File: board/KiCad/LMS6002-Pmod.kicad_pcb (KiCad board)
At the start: 2 copper layers, 30.5 x 29.2 mm, 3 parts, among them P1 PMOD_2x6, P2 PMOD_2x6, U1 iCE40_1K4K_TQ144

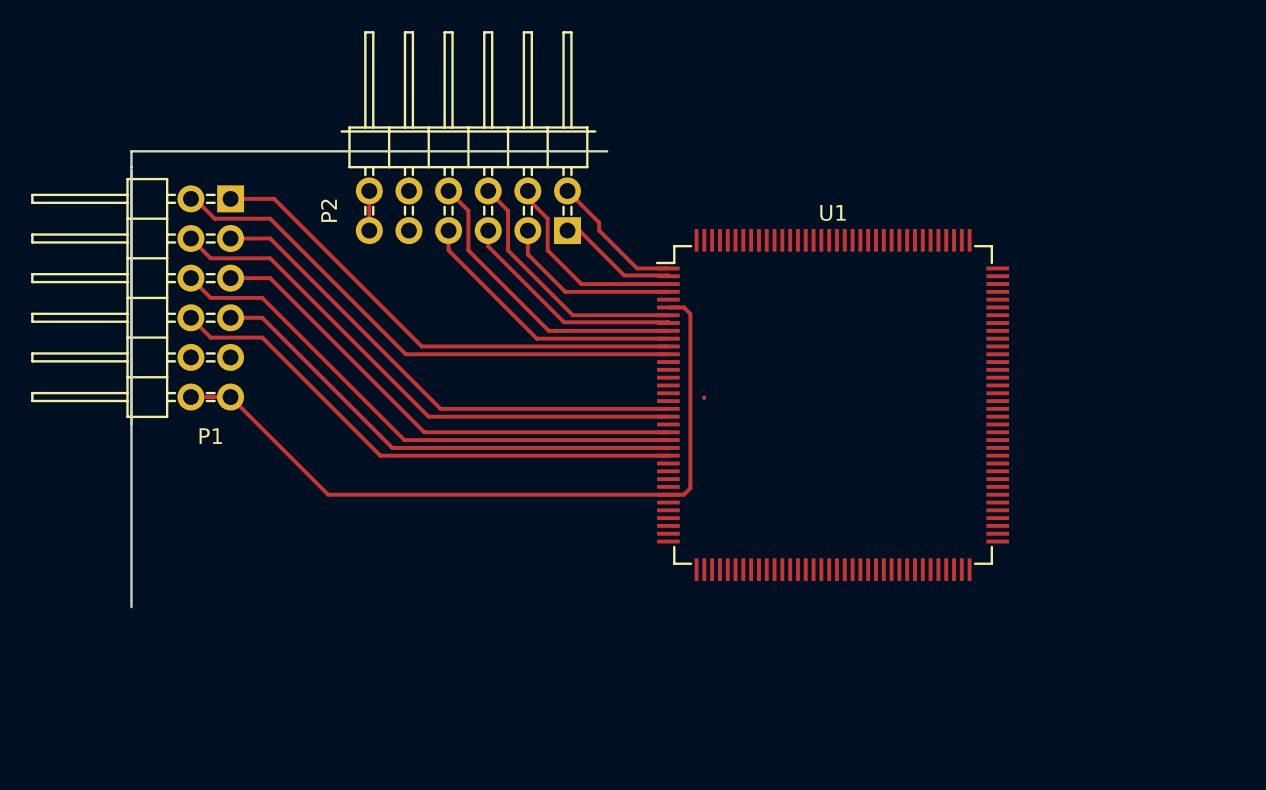
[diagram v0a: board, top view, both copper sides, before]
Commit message: Finalize first draft
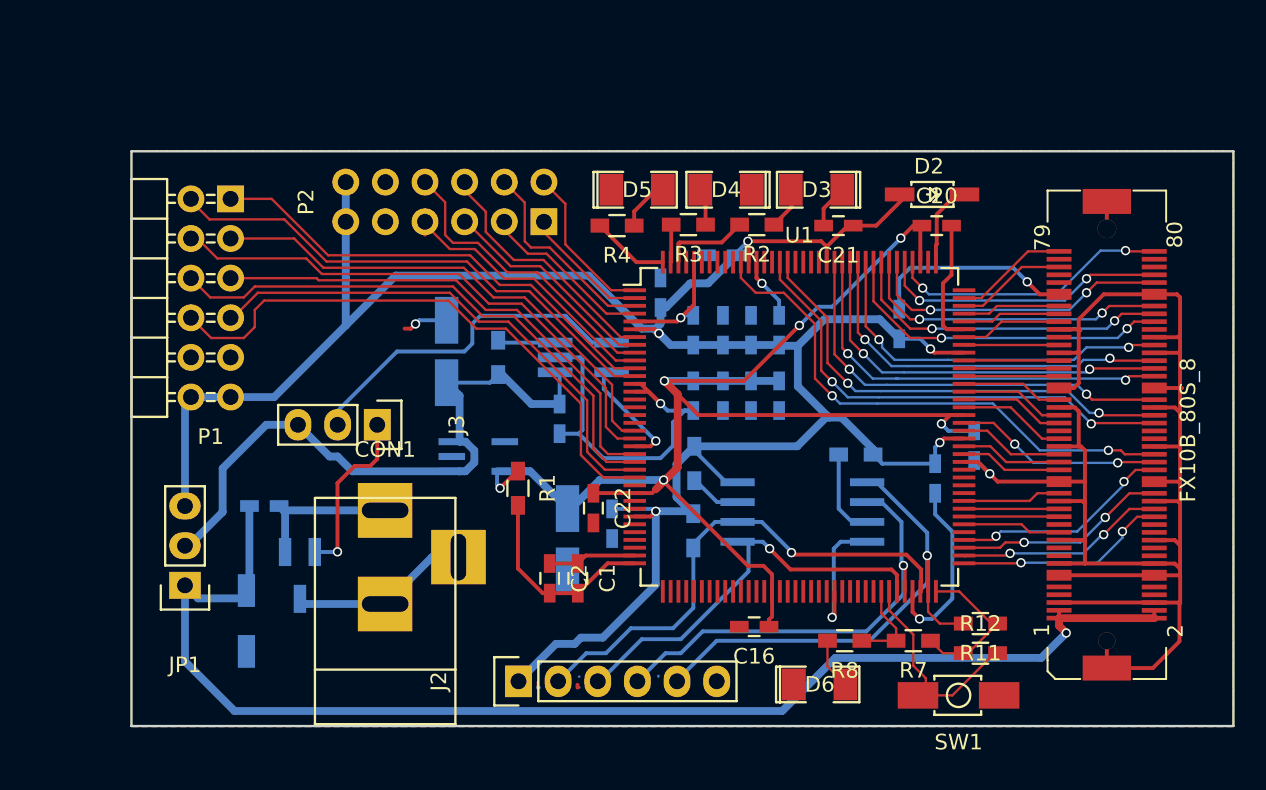
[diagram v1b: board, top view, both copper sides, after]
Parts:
- added C1: 10µF, Capacitors_SMD:C_0603_HandSoldering, F.Cu at (117.5, 112.2)
- added C10: 10µF, Capacitors_SMD:C_0603_HandSoldering, B.Cu at (126.8, 96.3)
- added C11: 1µF, Capacitors_SMD:C_0603_HandSoldering, B.Cu at (128.6, 96.3)
- added C12: 0.1µF, Capacitors_SMD:C_0603_HandSoldering, B.Cu at (130.4, 96.3)
- added C13: 0.01µF, Capacitors_SMD:C_0603_HandSoldering, B.Cu at (124.9, 96.3)
- added C14: 100n, Capacitors_SMD:C_0603_HandSoldering, B.Cu at (140.4, 105.8)
- added C15: 100n, Capacitors_SMD:C_0603_HandSoldering, B.Cu at (122.8, 93.9)
- added C16: 100n, Capacitors_SMD:C_0603_HandSoldering, F.Cu at (128.8, 115.3)
- added C17: 100n, Capacitors_SMD:C_0603_HandSoldering, B.Cu at (119.7, 108.7)
- added C18: 100n, Capacitors_SMD:C_0603_HandSoldering, B.Cu at (142.9, 103.7)
- added C19: 100n, Capacitors_SMD:C_0603_HandSoldering, B.Cu at (138.1, 95.9)
- added C2: 0.1µF, Capacitors_SMD:C_0603_HandSoldering, F.Cu at (115.7, 112.2)
- added C20: 100n, Capacitors_SMD:C_0603_HandSoldering, F.Cu at (140.5, 89.6)
- added C21: 100n, Capacitors_SMD:C_0603_HandSoldering, F.Cu at (134.2, 89.6)
- added C22: 100n, Capacitors_SMD:C_0603_HandSoldering, F.Cu at (118.5, 107.7)
- added C23: 100n, Capacitors_SMD:C_0603_HandSoldering, B.Cu at (126.7, 91.5)
- added C3: 1µF, Capacitors_Tantalum_SMD:TantalC_SizeA_EIA-3216_HandSoldering, B.Cu at (109.1, 97.7)
- added C4: 1µF, Capacitors_Tantalum_SMD:TantalC_SizeA_EIA-3216_HandSoldering, B.Cu at (116.8, 109.7)
- added C5: 0.1µ, Capacitors_SMD:C_0603_HandSoldering, B.Cu at (116.3, 102.0)
- added C6: 10µF, Capacitors_SMD:C_0603_HandSoldering, B.Cu at (126.8, 100.5)
- added C7: 1µF, Capacitors_SMD:C_0603_HandSoldering, B.Cu at (128.6, 100.5)
- added C8: 0.1µF, Capacitors_SMD:C_0603_HandSoldering, B.Cu at (124.9, 100.5)
- added C9: 0.01µF, Capacitors_SMD:C_0603_HandSoldering, B.Cu at (130.4, 100.5)
- added CON1: BARREL_JACK, Connect:BARREL_JACK, F.Cu at (105.2, 114.0)
- added D1: 5V-SOD-123F, pmod:SOD-123F_Handsoldering, B.Cu at (96.3, 114.9)
- added D2: Schottky 0520, pmod:SOD-123_Handsoldering, F.Cu at (140.2, 87.6)
- added D3: LED, SMD_Packages:SMD-1206_Pol, F.Cu at (132.8, 87.3)
- added D4: LED, SMD_Packages:SMD-1206_Pol, F.Cu at (127.0, 87.3)
- added D5: LED, SMD_Packages:SMD-1206_Pol, F.Cu at (121.3, 87.3)
- added D6: LED, SMD_Packages:SMD-1206_Pol, F.Cu at (133.0, 119.0)
- added F1: 2A-0603, Capacitors_SMD:C_0603_HandSoldering, B.Cu at (97.4, 107.6)
- added J1: FX10B_80S_8, pmod:FX10B_80S_8, F.Cu at (151.4, 103.0)
- added J2: Pinheader_1x6_TH, Pin_Headers:Pin_Header_Straight_1x06, F.Cu at (113.7, 118.8)
- added J3: SELECT_DIV, Pin_Headers:Pin_Header_Straight_1x03, F.Cu at (104.6, 102.4)
- added JP1: LDO_1V2_IN_SEL, Pin_Headers:Pin_Header_Straight_1x03, F.Cu at (92.3, 112.6)
- added Q1: IRLML6344bpf, TO_SOT_Packages_SMD:SOT-23_Handsoldering, B.Cu at (99.7, 112.0)
- added R1: 100, Resistors_SMD:R_0603_HandSoldering, F.Cu at (113.7, 106.4)
- added R10: 10k, Resistors_SMD:R_0603_HandSoldering, B.Cu at (135.3, 104.3)
- added R11: 10k, Resistors_SMD:R_0603_HandSoldering, F.Cu at (143.3, 115.1)
- added R12: 10K, Resistors_SMD:R_0603_HandSoldering, F.Cu at (143.3, 117.0)
- added R2: 10, Resistors_SMD:R_0603_HandSoldering, F.Cu at (129.0, 89.5)
- added R3: 10, Resistors_SMD:R_0603_HandSoldering, F.Cu at (124.6, 89.5)
- added R4: 10, Resistors_SMD:R_0603_HandSoldering, F.Cu at (120.0, 89.6)
- added R5: R, Resistors_SMD:R_0603_HandSoldering, B.Cu at (112.4, 98.0)
- added R6: 10k, Resistors_SMD:R_0603_HandSoldering, B.Cu at (124.9, 109.2)
- added R7: 10K, Resistors_SMD:R_0603_HandSoldering, F.Cu at (139.0, 116.2)
- added R8: 10, Resistors_SMD:R_0603_HandSoldering, F.Cu at (134.6, 116.2)
- added R9: 10k, Resistors_SMD:R_0603_HandSoldering, B.Cu at (125.0, 104.8)
- added SW1: ICE_RESET, pmod:B3U-1000P_Handsoldering, F.Cu at (141.9, 119.7)
- added U2: LD6815, pmod:SOT-753_(TSOP-5)_Handsoldering, B.Cu at (111.1, 104.4)
- added U3: LTC1799, pmod:TSOT-23_Handsoldering, B.Cu at (117.9, 98.0)
- added U4: N25Q, pmod:SOP2-8_Handsoldering, B.Cu at (131.9, 108.0)
- moved U1 2.57 mm to (131.7, 102.5)
- moved P2 1.61 mm to (116.6, 83.0)
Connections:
- P1 pad 12: +3V3 -> 3V3_PMOD
- P1 pad 6: +3V3 -> 3V3_PMOD
- P2 pad 12: +3V3 -> 3V3_PMOD
- P2 pad 6: +3V3 -> 3V3_PMOD
- U1 pad 100: Net-(U1-Pad100) -> 3V3_PMOD
- U1 pad 101: Net-(U1-Pad101) -> FCLK2
- U1 pad 102: Net-(U1-Pad102) -> RFDIO_GPIO0
- U1 pad 103: Net-(U1-Pad103) -> GND
- U1 pad 104: Net-(U1-Pad104) -> RFDIO_GPIO1
- U1 pad 105: Net-(U1-Pad105) -> RFDIO_GPIO2
- U1 pad 106: Net-(U1-Pad106) -> RFDIO_REF_CLK_IN
- U1 pad 107: Net-(U1-Pad107) -> TXEN
- U1 pad 108: Net-(U1-Pad108) -> (no net)
- U1 pad 110: Net-(U1-Pad110) -> (no net)
- U1 pad 111: Net-(U1-Pad111) -> 1V2_LDO
- U1 pad 112: Net-(U1-Pad112) -> RXEN
- U1 pad 113: Net-(U1-Pad113) -> RFDIO_SPI_EN
- U1 pad 114: Net-(U1-Pad114) -> RFDIO_SPI_CLK
- U1 pad 115: Net-(U1-Pad115) -> RFDIO_SPI_MISO
- U1 pad 116: Net-(U1-Pad116) -> RFDIO_SPI_MOSI
- U1 pad 117: Net-(U1-Pad117) -> RFDIO_RESET
- U1 pad 118: Net-(U1-Pad118) -> FCLK1
- U1 pad 119: Net-(U1-Pad119) -> DIQ2_D11
- U1 pad 120: Net-(U1-Pad120) -> DIQ2_D9
- U1 pad 121: Net-(U1-Pad121) -> DIQ2_D7
- U1 pad 122: Net-(U1-Pad122) -> DIQ2_D5
- U1 pad 123: Net-(U1-Pad123) -> 3V3_PMOD
- U1 pad 124: Net-(U1-Pad124) -> (no net)
- U1 pad 125: Net-(U1-Pad125) -> (no net)
- U1 pad 126: Net-(U1-Pad126) -> (no net)
- U1 pad 127: Net-(U1-Pad127) -> (no net)
- U1 pad 128: Net-(U1-Pad128) -> DIQ2_D3
- U1 pad 129: Net-(U1-Pad129) -> DIQ2_D1
- U1 pad 13: Net-(U1-Pad13) -> GND
- U1 pad 130: Net-(U1-Pad130) -> (no net)
- U1 pad 131: Net-(U1-Pad131) -> (no net)
- U1 pad 132: Net-(U1-Pad132) -> GND
- U1 pad 133: Net-(U1-Pad133) -> 3V3_PMOD
- U1 pad 134: Net-(U1-Pad134) -> DIQ1_D11
- U1 pad 135: Net-(U1-Pad135) -> (no net)
- U1 pad 136: Net-(U1-Pad136) -> (no net)
- U1 pad 137: Net-(U1-Pad137) -> (no net)
- U1 pad 138: Net-(U1-Pad138) -> (no net)
- U1 pad 139: Net-(U1-Pad139) -> (no net)
- U1 pad 14: Net-(U1-Pad14) -> GND
- U1 pad 140: Net-(U1-Pad140) -> GND
- U1 pad 141: Net-(U1-Pad141) -> (no net)
- U1 pad 15: Net-(U1-Pad15) -> (no net)
- U1 pad 16: Net-(U1-Pad16) -> (no net)
- U1 pad 17: Net-(U1-Pad17) -> (no net)
- U1 pad 18: Net-(U1-Pad18) -> (no net)
- U1 pad 21: Net-(U1-Pad21) -> ICE_CLK_IN
- U1 pad 26: Net-(U1-Pad26) -> (no net)
- U1 pad 27: Net-(U1-Pad27) -> 1V2_LDO
- U1 pad 28: Net-(U1-Pad28) -> (no net)
- U1 pad 29: Net-(U1-Pad29) -> (no net)
- U1 pad 30: +3V3 -> 3V3_PMOD
- U1 pad 31: Net-(U1-Pad31) -> (no net)
- U1 pad 32: Net-(U1-Pad32) -> (no net)
- U1 pad 33: Net-(U1-Pad33) -> (no net)
- U1 pad 34: Net-(U1-Pad34) -> (no net)
- U1 pad 37: Net-(U1-Pad37) -> (no net)
- U1 pad 38: Net-(U1-Pad38) -> (no net)
- U1 pad 39: Net-(U1-Pad39) -> (no net)
- U1 pad 40: Net-(U1-Pad40) -> (no net)
- U1 pad 41: Net-(U1-Pad41) -> (no net)
- U1 pad 42: Net-(U1-Pad42) -> (no net)
- U1 pad 43: Net-(U1-Pad43) -> (no net)
- U1 pad 44: Net-(U1-Pad44) -> (no net)
- U1 pad 45: Net-(U1-Pad45) -> (no net)
- U1 pad 46: Net-(U1-Pad46) -> (no net)
- U1 pad 47: Net-(U1-Pad47) -> (no net)
- U1 pad 48: Net-(U1-Pad48) -> (no net)
- U1 pad 49: Net-(U1-Pad49) -> (no net)
- U1 pad 5: Net-(U1-Pad5) -> GND
- U1 pad 50: Net-(U1-Pad50) -> (no net)
- U1 pad 51: Net-(U1-Pad51) -> 1V2_LDO
- U1 pad 52: Net-(U1-Pad52) -> (no net)
- U1 pad 53: Net-(U1-Pad53) -> (no net)
- U1 pad 54: Net-(U1-Pad54) -> (no net)
- U1 pad 55: Net-(U1-Pad55) -> (no net)
- U1 pad 56: Net-(U1-Pad56) -> (no net)
- U1 pad 57: Net-(U1-Pad57) -> (no net)
- U1 pad 58: Net-(U1-Pad58) -> (no net)
- U1 pad 59: Net-(U1-Pad59) -> GND
- U1 pad 6: +3V3 -> 3V3_PMOD
- U1 pad 60: Net-(U1-Pad60) -> (no net)
- U1 pad 61: Net-(U1-Pad61) -> (no net)
- U1 pad 62: Net-(U1-Pad62) -> (no net)
- U1 pad 63: Net-(U1-Pad63) -> (no net)
- U1 pad 64: Net-(U1-Pad64) -> (no net)
- U1 pad 65: Net-(U1-Pad65) -> ICE_CDONE
- U1 pad 66: Net-(U1-Pad66) -> ICE_CRESET_B
- U1 pad 67: Net-(U1-Pad67) -> EXT_SPI_MOSI
- U1 pad 68: Net-(U1-Pad68) -> EXT_SPI_MISO
- U1 pad 69: Net-(U1-Pad69) -> GND
- U1 pad 70: Net-(U1-Pad70) -> EXT_SPI_CLK
- U1 pad 71: Net-(U1-Pad71) -> EXT_SPI_SS_B
- U1 pad 72: Net-(U1-Pad72) -> 3V3_PMOD
- U1 pad 73: Net-(U1-Pad73) -> DIQ1_D1
- U1 pad 74: Net-(U1-Pad74) -> DIQ1_D3
- U1 pad 75: Net-(U1-Pad75) -> DIQ1_D5
- U1 pad 76: Net-(U1-Pad76) -> DIQ1_D7
- U1 pad 77: Net-(U1-Pad77) -> (no net)
- U1 pad 78: Net-(U1-Pad78) -> DIQ1_SEL
- U1 pad 79: Net-(U1-Pad79) -> DIQ1_D0
- U1 pad 80: Net-(U1-Pad80) -> DIQ1_D2
- U1 pad 81: Net-(U1-Pad81) -> DIQ1_D4
- U1 pad 82: Net-(U1-Pad82) -> (no net)
- U1 pad 83: Net-(U1-Pad83) -> (no net)
- U1 pad 84: Net-(U1-Pad84) -> (no net)
- U1 pad 85: Net-(U1-Pad85) -> (no net)
- U1 pad 86: Net-(U1-Pad86) -> GND
- U1 pad 87: Net-(U1-Pad87) -> DIQ1_D6
- U1 pad 88: Net-(U1-Pad88) -> DIQ1_D8
- U1 pad 89: Net-(U1-Pad89) -> 3V3_PMOD
- U1 pad 90: Net-(U1-Pad90) -> DIQ1_D10
- U1 pad 91: Net-(U1-Pad91) -> DIQ1_D9
- U1 pad 92: Net-(U1-Pad92) -> 1V2_LDO
- U1 pad 93: Net-(U1-Pad93) -> DIQ2_SEL
- U1 pad 94: Net-(U1-Pad94) -> DIQ2_D0
- U1 pad 95: Net-(U1-Pad95) -> DIQ2_D2
- U1 pad 96: Net-(U1-Pad96) -> DIQ2_D4
- U1 pad 97: Net-(U1-Pad97) -> DIQ2_D6
- U1 pad 98: Net-(U1-Pad98) -> DIQ2_D8
- U1 pad 99: Net-(U1-Pad99) -> DIQ2_D10
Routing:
- net GND: track 0.00 -> 204.9 mm, vias 0 -> 9
- net 3V3_PMOD: track 0.00 -> 178.9 mm, vias 0 -> 5
- net 1V2_LDO: track 0.00 -> 94.5 mm, vias 0 -> 6
- net 5V: track 0.00 -> 83.3 mm, vias 0 -> 1
- net +3V3: track 50.1 -> 0.00 mm
- net 5V_LDO_IN: track 0.00 -> 41.5 mm
- net DIQ1_D11: track 0.00 -> 34.2 mm, vias 0 -> 2
- net EXT_SPI_SS_B: track 0.00 -> 34.0 mm, vias 0 -> 1
- net EXT_SPI_CLK: track 0.00 -> 32.7 mm, vias 0 -> 1
- net DIQ2_D1: track 0.00 -> 30.8 mm, vias 0 -> 2
- net EXT_SPI_MISO: track 0.00 -> 30.8 mm, vias 0 -> 1
- net DIQ2_D3: track 0.00 -> 29.8 mm, vias 0 -> 2
- net DIQ2_D5: track 0.00 -> 27.6 mm, vias 0 -> 2
- net DIQ2_D7: track 0.00 -> 26.6 mm, vias 0 -> 2
- net EXT_SPI_MOSI: track 0.00 -> 26.3 mm, vias 0 -> 1
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- added copper zone on B.Cu, net GND
- added copper zone on F.Cu, net GND
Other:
- board size 30.5 x 29.2 mm -> 70.6 x 36.8 mm
- net class Default: clearance 0.2 -> 0.1524
- net class SeeedMinimum added: clearance 0.1524, trace_width 0.1524, via_dia 0.6, via_drill 0.3
- rule trace_clearance: 0.2 -> 0.1524
- rule trace_min: 0.2 -> 0.1524
